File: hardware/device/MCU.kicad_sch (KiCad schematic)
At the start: 20 parts, among them J4 EXPANSION, SW24 NRST, U18 STM32H743ZIT6

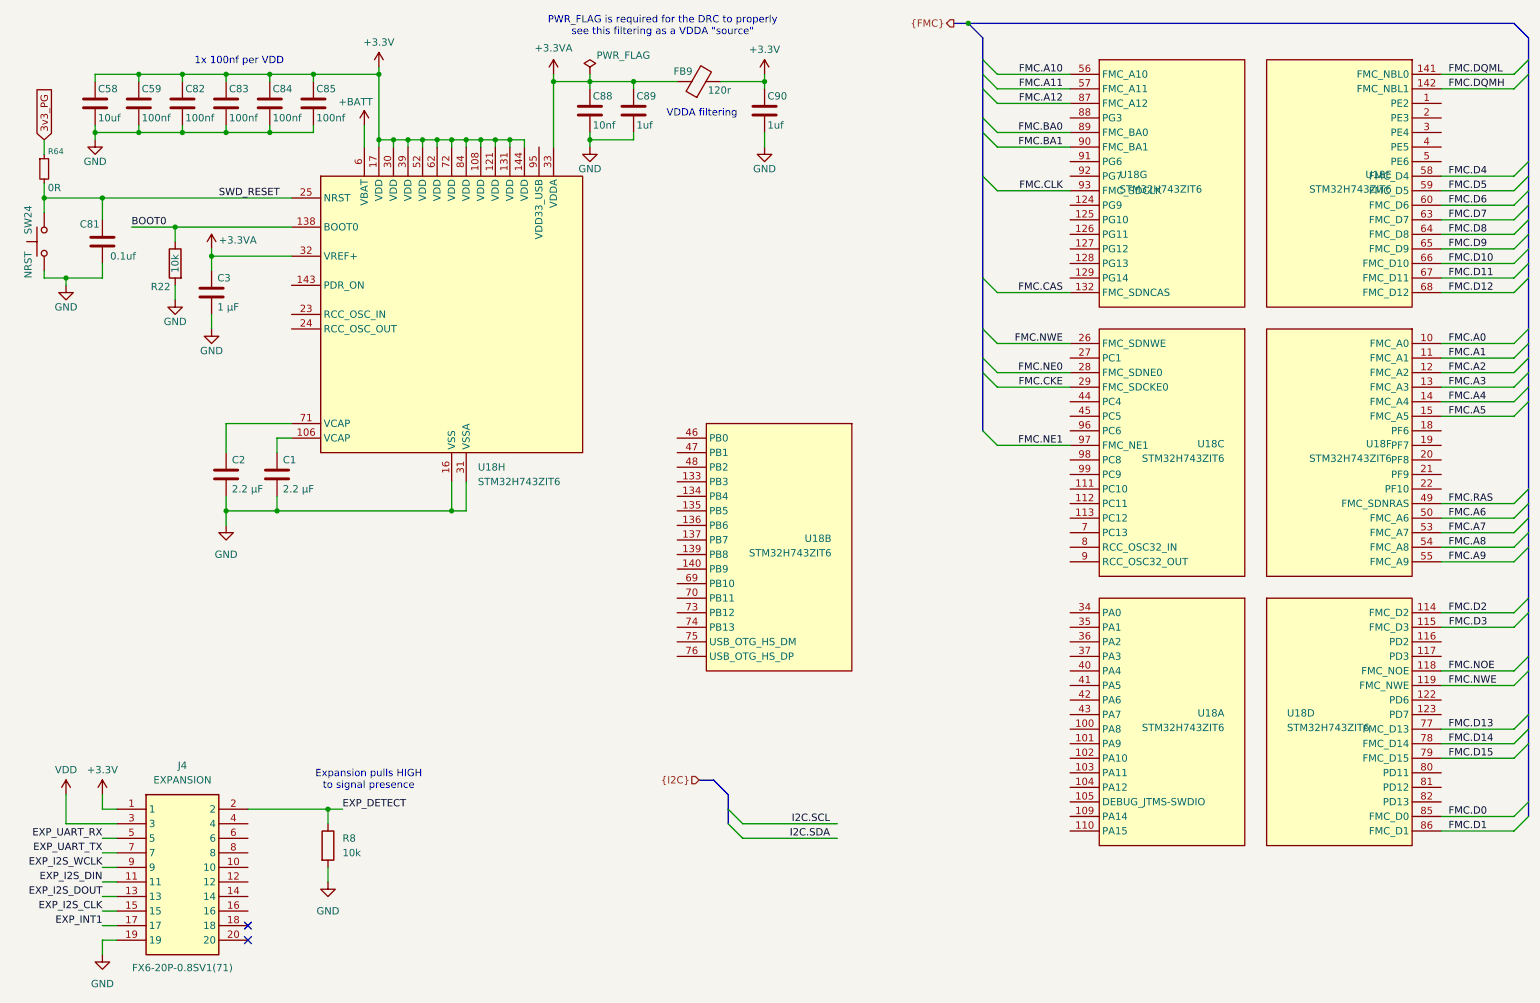
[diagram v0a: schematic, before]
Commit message: feat: various layouts, changed SDRAM to BGA
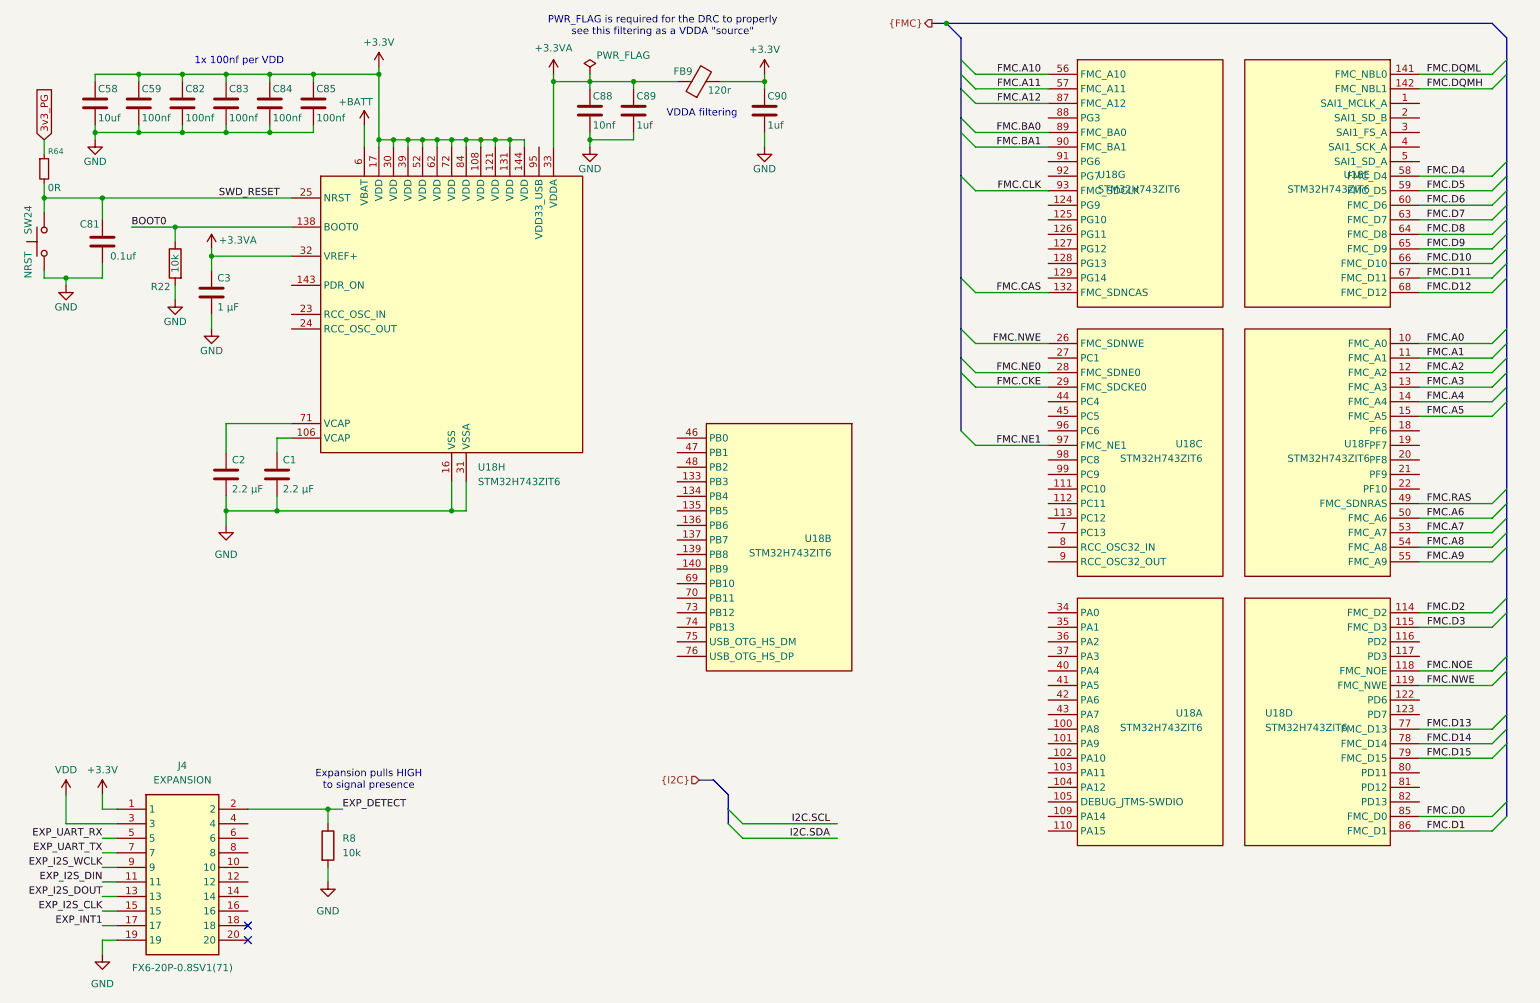
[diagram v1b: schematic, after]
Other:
- moved on the sheet: U18A, U18C, U18D, U18E, U18F, U18G
